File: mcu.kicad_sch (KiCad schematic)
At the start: 88 parts, among them U1 PIC32CK1025GC01100-I/4SB

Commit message: did alot of stuff
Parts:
- removed TP2, TP23, TP24, TP25 (x2), TP3, TP36, TP39: TestPoint, symbol Connector:TestPoint
- removed U1: PIC32CK1025GC01100-I/4SB, PIC32CK1025GC01100-I-4SB:TQFP100_4SB_6p3EP_MCH, symbol PIC32CK1025GC01100-I-4SB:PIC32CK1025GC01100-I_4SB
- added C1, C10, C11, C12, C14, C16, C2, C3, C4, C5, C6, C7, C8: 100n, Capacitor_SMD:C_0402_1005Metric, symbol Device:C
- added C13, C18, C9: 47u, Capacitor_SMD:C_1210_3225Metric, symbol Device:C
- added C15: 4.7u, Capacitor_SMD:C_0805_2012Metric, symbol Device:C
- added C17: 10u, Capacitor_SMD:C_0805_2012Metric, symbol Device:C
- added C19, C20, C21, C22: C, Capacitor_SMD:C_0402_1005Metric, symbol Device:C
- added D1, D2: LED, LED_SMD:LED_0805_2012Metric, symbol Device:LED
- added FB2: FerriteBead_Small, symbol Device:FerriteBead_Small
- added Q1, Q2: NMOS, symbol Simulation_SPICE:NMOS
- added R1, R2: 0, Resistor_SMD:R_0402_1005Metric, symbol Device:R
- added R3, R4: R, Resistor_SMD:R_0402_1005Metric, symbol Device:R
- added R5, R6, R8, R9: 10k, Resistor_SMD:R_0402_1005Metric, symbol Device:R
- added R7: 270, Resistor_SMD:R_0402_1005Metric, symbol Device:R
- added SW1: SW_Push, symbol Switch:SW_Push
- added TP43, TP45, TP46: TestPoint, symbol Connector:TestPoint
- added unit 2 of U1
- added Y1, Y2: Crystal, symbol Device:Crystal
- renumbered TP4 to TP47, TP5 to TP48, TP6 to TP49, TP7 to TP50, TP8 to TP51, TP9 to TP52, TP10 to TP53, TP11 to TP54, TP12 to TP55, TP13 to TP56, TP14 to TP57, TP15 to TP58, TP16 to TP59, TP17 to TP60, TP18 to TP61, TP19 to TP62, TP20 to TP63, TP21 to TP64, TP22 to TP65, TP23 to TP66, TP26 to TP67, TP27 to TP68, TP28 to TP69, TP29 to TP70, TP30 to TP71, TP31 to TP72, TP32 to TP73, TP33 to TP74, TP34 to TP75, TP35 to TP76, TP37 to TP77, TP38 to TP78, TP40 to TP79, TP41 to TP80, TP42 to TP81, TP1 to TP82, TP43 to TP83
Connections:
- net +3.3V: now also C1.1, C10.1, C11.1, C12.1, C13.1, C14.1, C15.1, C18.1, C2.1, C3.1, C4.1, C5.1, C6.1, C7.1, C8.1, C9.1, FB2.1, R3.1, R4.1, R5.1, R9.1, SW1.1, U1.20 (VDDIO), U1.34 (VDDIO), U1.42 (VDDIO), U1.44 (VDDREG), U1.56 (VDDIO), U1.62 (VDDREG), U1.69 (VDDIO), U1.7 (VDDIO), U1.79 (VCCAP3), U1.83 (VDDREG), U1.85 (VDDIO), U1.96 (VDDIO)
- net GND: now also C1.2, C10.2, C11.2, C12.2, C13.2, C14.2, C15.2, C16.2, C17.2, C18.2, C19.2, C2.2, C20.2, C21.2, C22.2, C3.2, C4.2, C5.2, C6.2, C7.2, C8.2, C9.2, D2.1 (K), Q1.3 (S), Q2.3 (S), R6.2, R7.2, R8.2, U1.101 (GND), U1.19 (GND), U1.30 (VSSA), U1.35 (GND), U1.43 (GND), U1.57 (GND), U1.6 (GND), U1.70 (GND), U1.80 (USBVSSA), U1.84 (VSSIO), U1.95 (GND)
- net SPARE1: no longer TP64.1, U1.45 (PB16)
- net SPARE10: no longer TP83.1, U1.82 (USRBIAS)
- net SPARE11: no longer TP44.1
- net SPARE2: no longer TP65.1, U1.46 (PB17)
- net SPARE4: no longer TP67.1, U1.87 (PD01)
- net SPARE5: no longer TP68.1, U1.88 (PD02)
- net SPARE6: no longer TP69.1, U1.92 (PD05)
- net SPARE7: no longer TP70.1, U1.93 (PD06)
- net SPARE8: no longer TP71.1, U1.94 (PD07)
- net SPARE9: no longer TP78.1, U1.90 (USB_DP)
- net SPI2.CS#: no longer TP81.1, U1.77 (USB0PP)
- net SPI2.MISO: no longer TP79.1, U1.78 (USB0ID)
- net SPI2.SCK: no longer TP80.1, U1.76 (USB0PN)
- net SPI5.CS#: no longer TP63.1, U1.41 (PB15)
- net SPI5.MISO: no longer TP61.1, U1.38 (PB13)
- net SPI5.MOSI: no longer TP60.1, U1.29 (PB12)
- net SPI5.SCK: no longer TP62.1, U1.40 (PB14)
- net SPI6.CS#: no longer TP57.1, U1.49 (PB09)
- net SPI6.MISO: no longer TP55.1, U1.47 (PB07)
- net SPI6.MOSI: no longer TP54.1, U1.39 (PB06)
- net SPI6.SCK: no longer TP56.1, U1.48 (PB08)
- net SPI7.MISO: now also TP5.1, U1.13 (PA04); no longer TP52.1, TP6.1, U1.14 (PA05), U1.36 (PB04)
- net SPI7.MOSI: now also R1.2; no longer TP5.1, TP51.1, U1.13 (PA04), U1.32 (PB03)
- net SPI7.SCK: now also TP6.1, U1.14 (PA05); no longer TP53.1, TP7.1, U1.15 (PA06), U1.37 (PB05)
- net SPARE12: now reaches TP47.1, TP48.1, U1.26 (PB00)
- net PA01: now reaches TP2.1, TP21.1, U1.2 (PA01)
- net PA01: now also R1.1, R2.1
- net JTAG.TDI: now reaches TP1.1, TP20.1, U1.1 (PA00)
- net EXT: now reaches U1.21 (EXT)
- net EXT: now also TP45.1, TP46.1
- net RESET#: now reaches U1.5 (RESET_N)
- net RESET#: now also TP44.1, Q2.1 (D), R5.2, TP43.1
- net ETH.MDC renamed SMI.MDC
- net SMI.MDC: no longer TP58.1, U1.50 (PB10)
- net ETH.MDIO renamed ADC_VINP10
- net ADC_VINP10: no longer TP13.1, U1.25 (PA12)
- net ETH.RXD0 renamed RMII.RXD0
- net RMII.RXD0: no longer TP73.1, U1.98 (PD09)
- net ETH.RXD1 renamed RMII.RXD1
- net RMII.RXD1: no longer TP72.1, U1.97 (PD08)
- net ETH.RXDV renamed RMII.CRSDV
- net RMII.CRSDV: no longer TP75.1, U1.100 (PD11)
- net ETH.RXER renamed RMII.RXER
- net RMII.RXER: no longer TP74.1, U1.99 (PD10)
- net ETH.TXD0 renamed RMII.TXD0
- net ETH.TXD1 renamed RMII.TXD1
- net RMII.TXD1: no longer TP77.1, U1.89 (USB_DM)
- net ETH.TXEN renamed RMII.TXEN
- net RMII.TXEN: no longer TP76.1, U1.91 (PD12)
- net SPARE3 renamed RMII.REFCK
- net RMII.REFCK: no longer TP66.1, U1.86 (PD00)
- net SWD.SWCLK renamed JTAG.TCK
- net JTAG.TCK: no longer TP50.1, U1.31 (PB02)
- net SWD.SWDIO renamed JTAG.TMS
- net JTAG.TMS: no longer TP49.1, U1.27 (PB01)
- new net: C16.1, C17.1, FB2.2, U1.33 (VDDA)
- new net: D1.2 (A), R3.2
- new net: D1.1 (K), Q1.1 (D)
- new net: D2.2 (A), R4.2
- new net ADC_VINP11: TP60.1, U1.29 (PB12)
- new net JTAG.TDO: R2.2
- new net RST_BTN: Q2.2 (G), R6.1, SW1.2
- new net SDMMC0_SDCD: TP76.1, U1.91 (PD12)
- new net SDMMC0_SDCK: TP74.1, U1.99 (PD10)
- new net SDMMC0_SDCMD: TP70.1, U1.93 (PD06)
- new net SDMMC0_SDDAT0: TP71.1, U1.94 (PD07)
- new net SDMMC0_SDDAT1: TP75.1, U1.100 (PD11)
- new net SDMMC0_SDDAT2: TP72.1, U1.97 (PD08)
- new net SDMMC0_SDDAT3: TP73.1, U1.98 (PD09)
- new net SDMMC0_SDWP: TP69.1, U1.92 (PD05)
- new net SMI.MDIO: TP13.1, U1.25 (PA12)
- new net SPARE13: TP49.1, U1.27 (PB01)
- new net SPARE14: TP57.1, U1.49 (PB09)
- new net SPARE15: TP58.1, U1.50 (PB10)
- new net SPARE16: TP62.1, U1.40 (PB14)
- new net SPARE17: TP63.1, U1.41 (PB15)
- new net SPI3.CS#: TP56.1, U1.48 (PB08)
- new net SPI3.MISO: TP65.1, U1.46 (PB17)
- new net SPI3.MOSI: TP64.1, U1.45 (PB16)
- new net SPI3.SCK: TP55.1, U1.47 (PB07)
- new net SPI4.CS#: TP54.1, U1.39 (PB06)
- new net SPI4.MISO: TP53.1, U1.37 (PB05)
- new net SPI4.MOSI: TP52.1, U1.36 (PB04)
- new net SPI4.SCK: TP61.1, U1.38 (PB13)
- new net SPI7.CS#: TP7.1, U1.15 (PA06)
- new net STATUS_LED: Q1.2 (G)
- new net TSUCOMP: TP68.1, U1.88 (PD02)
- new net USB0ID: R8.1, R9.2, TP79.1, U1.78 (USB0ID)
- new net USB_FS.D+: TP78.1, U1.90 (USB_DP)
- new net USB_FS.D-: TP77.1, U1.89 (USB_DM)
- new net USB_HS.D+: TP81.1, U1.77 (USB0PP)
- new net USB_HS.D-: TP80.1, U1.76 (USB0PN)
- new net USRBIAS: R7.1, TP83.1, U1.82 (USRBIAS)
- new net XIN: C19.1, TP66.1, U1.86 (PD00), Y1.1
- new net XIN32: C22.1, TP50.1, U1.31 (PB02), Y2.1
- new net XOUT: C21.1, TP67.1, U1.87 (PD01), Y1.2
- new net XOUT32: C20.1, TP51.1, U1.32 (PB03), Y2.2
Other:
- note added: "DNM"
- note added: "Design Note: 24 KHz 8pF 10ppm Crystal"
- note added: "Design Note: 32.768 KHz 10pF 10ppm Crystal"
- note added: "Design Note: Force USB OTG to Device role"
- note added: "Design Note: TSUCOMP compares PTP time to value option to trigger ADC perhaps"
- note added: "Microcontroller"
- moved on the sheet: TP1, TP10, TP11, TP12, TP13, TP14, TP15, TP16, TP17, TP18, TP19, TP2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

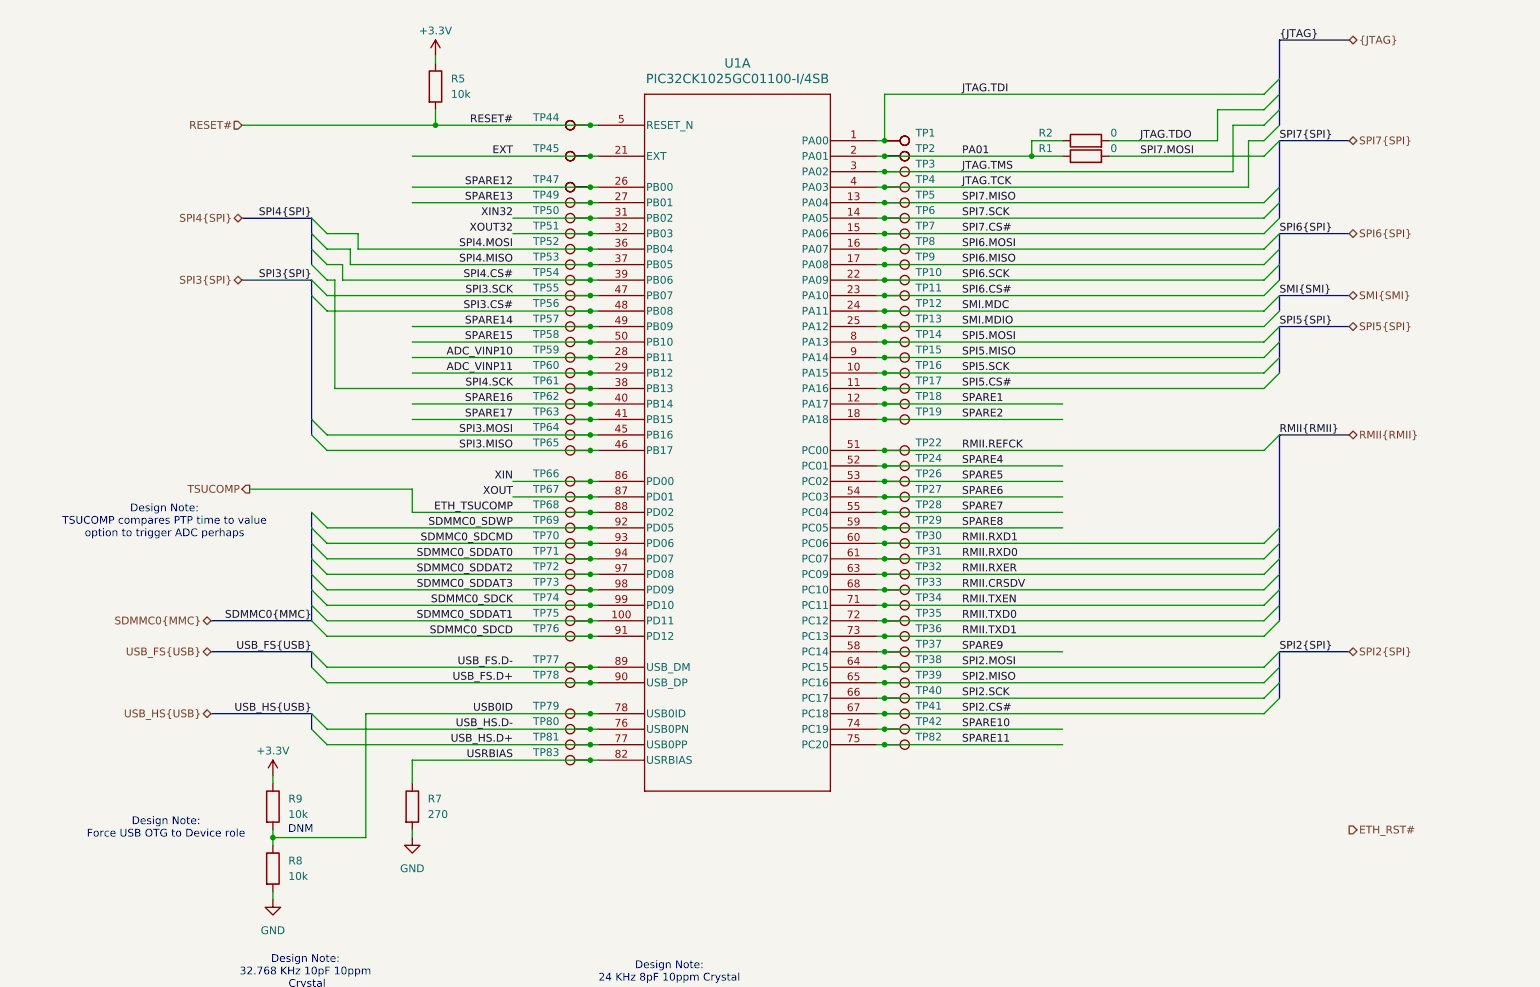
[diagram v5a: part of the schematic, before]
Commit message: stuff
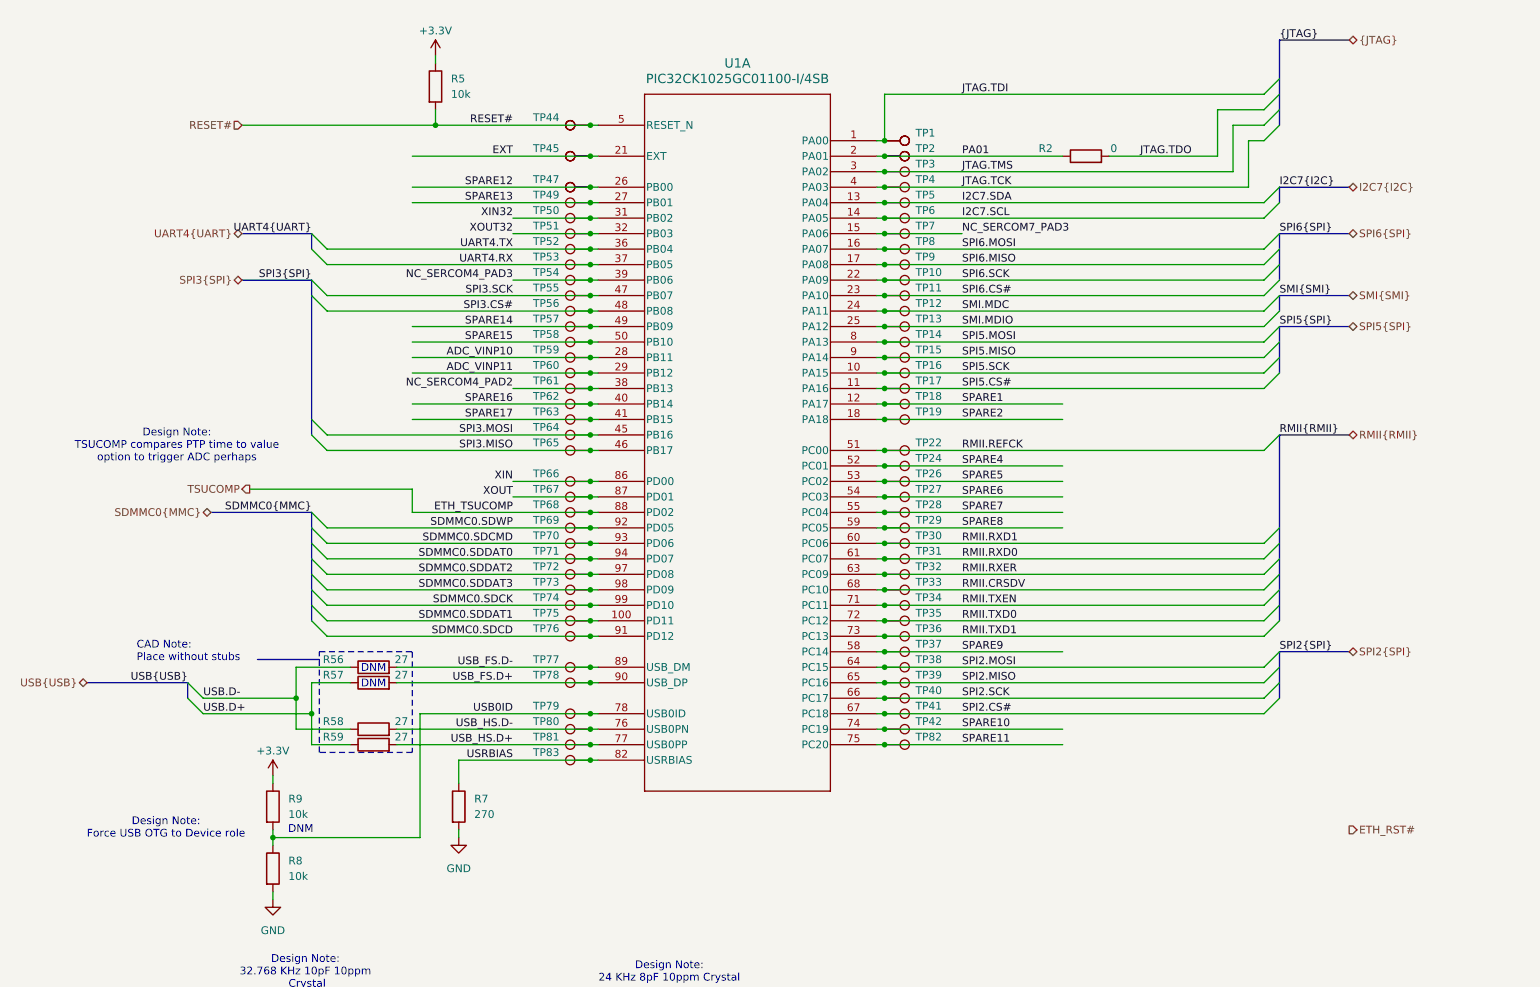
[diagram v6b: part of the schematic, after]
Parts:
- removed R1: 0, Resistor_SMD:R_0402_1005Metric, symbol Device:R
- added R56, R57, R58, R59: 27, Resistor_SMD:R_0402_1005Metric, symbol Device:R
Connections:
- net USB_FS.D+: now also R57.2
- net USB_FS.D-: now also R56.2
- net USB_HS.D+: now also R59.2
- net USB_HS.D-: now also R58.2
- net SDMMC0_SDCD renamed SDMMC0.SDCD
- net SDMMC0_SDCK renamed SDMMC0.SDCK
- net SDMMC0_SDCMD renamed SDMMC0.SDCMD
- net SDMMC0_SDDAT0 renamed SDMMC0.SDDAT0
- net SDMMC0_SDDAT1 renamed SDMMC0.SDDAT1
- net SDMMC0_SDDAT2 renamed SDMMC0.SDDAT2
- net SDMMC0_SDDAT3 renamed SDMMC0.SDDAT3
- net SDMMC0_SDWP renamed SDMMC0.SDWP
- net SPI4.CS# renamed NC_SERCOM4_PAD3
- net SPI4.MISO renamed UART4.RX
- net SPI4.MOSI renamed UART4.TX
- net SPI4.SCK renamed NC_SERCOM4_PAD2
- net SPI7.CS# renamed NC_SERCOM7_PAD3
- net SPI7.MISO renamed I2C7.SDA
- net SPI7.SCK renamed I2C7.SCL
- new net USB.D+: R57.1, R59.1
- new net USB.D-: R56.1, R58.1
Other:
- note added: "CAD Note: Place without stubs"
- moved on the sheet: R2, R7
